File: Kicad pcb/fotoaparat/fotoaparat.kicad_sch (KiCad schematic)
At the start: 75 parts, among them IC1 Lineární Regulátor, IC3 Lineární Regulátor Displaye, J1 USB Konektor, J2 SWD, J3 LCD konektor, J4 Baterie, J5 GSD090012SEU, J6 UART, J7 Kamera, J9 Conn_01x11_Socket, U1 STM32L496RETx, U2 MCP73833-FCI/UN, Y1 8mhz krystal

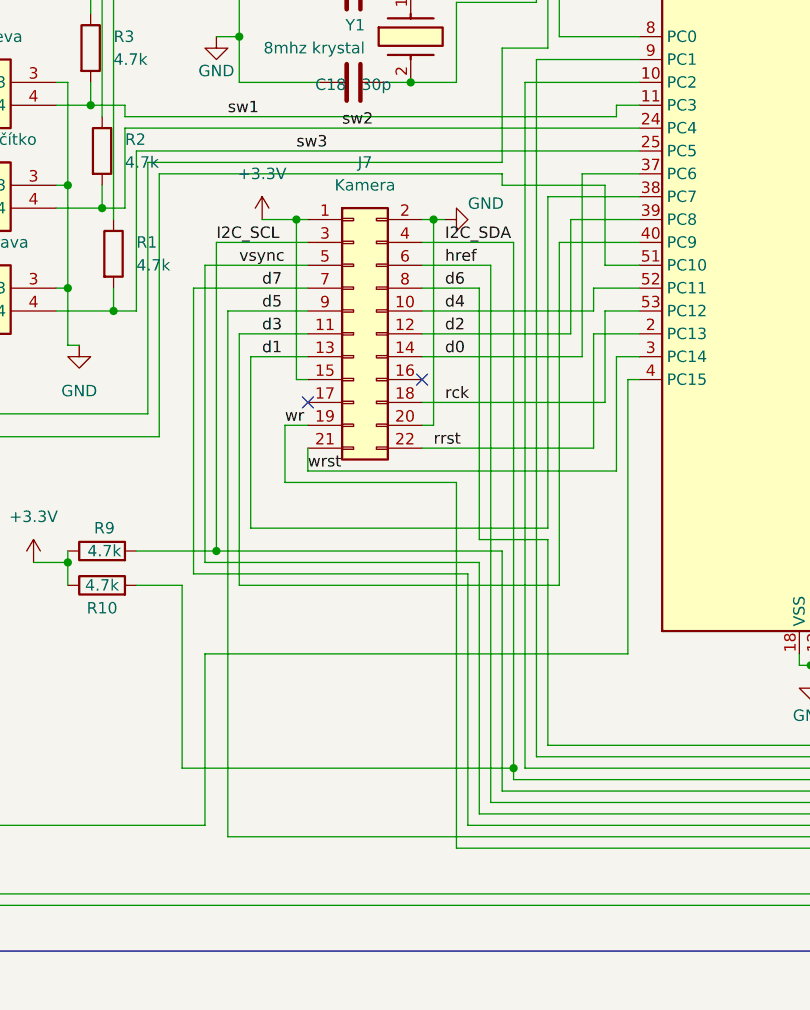
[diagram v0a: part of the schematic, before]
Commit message: Příprava na výrobu pcb
Gerber soubory se pravděpodobně ještě změní
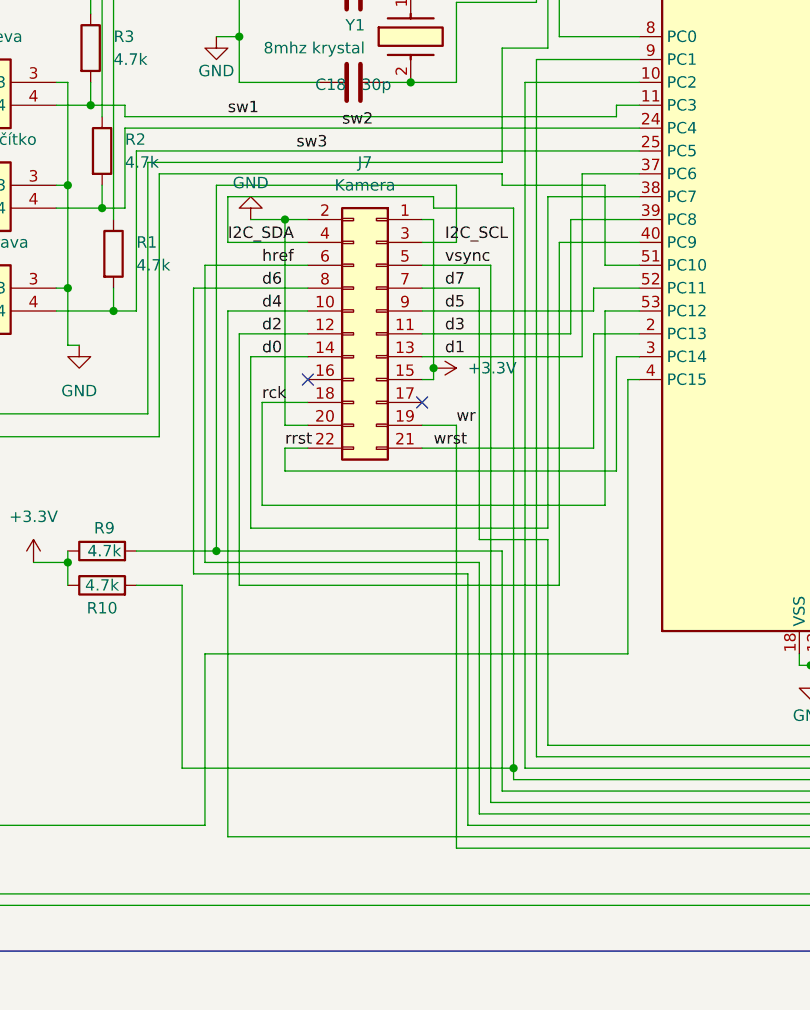
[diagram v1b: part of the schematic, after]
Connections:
- net d0: now also U1.38 (PC7); no longer U1.37 (PC6)
- net d1: now also U1.37 (PC6); no longer U1.38 (PC7)
- net d2: now also U1.40 (PC9); no longer U1.39 (PC8)
- net d3: now also U1.39 (PC8); no longer U1.40 (PC9)
- net d4: now also U1.58 (PB6); no longer U1.52 (PC11)
- net d5: now also U1.52 (PC11); no longer U1.58 (PB6)
- net d6: now also U1.62 (PB9); no longer U1.61 (PB8)
- net d7: now also U1.61 (PB8); no longer U1.62 (PB9)
- net href: now also U1.59 (PB7); no longer U1.20 (PA4)
- net rrst: now also U1.3 (PC14); no longer U1.2 (PC13)
- net vsync: now also U1.20 (PA4); no longer U1.59 (PB7)
- net wrst: now also U1.2 (PC13); no longer U1.3 (PC14)
